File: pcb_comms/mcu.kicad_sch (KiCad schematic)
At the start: 24 parts, among them SW1 SW_SPDT, U3 STM32WLE5CCU6, Y2 32MHz

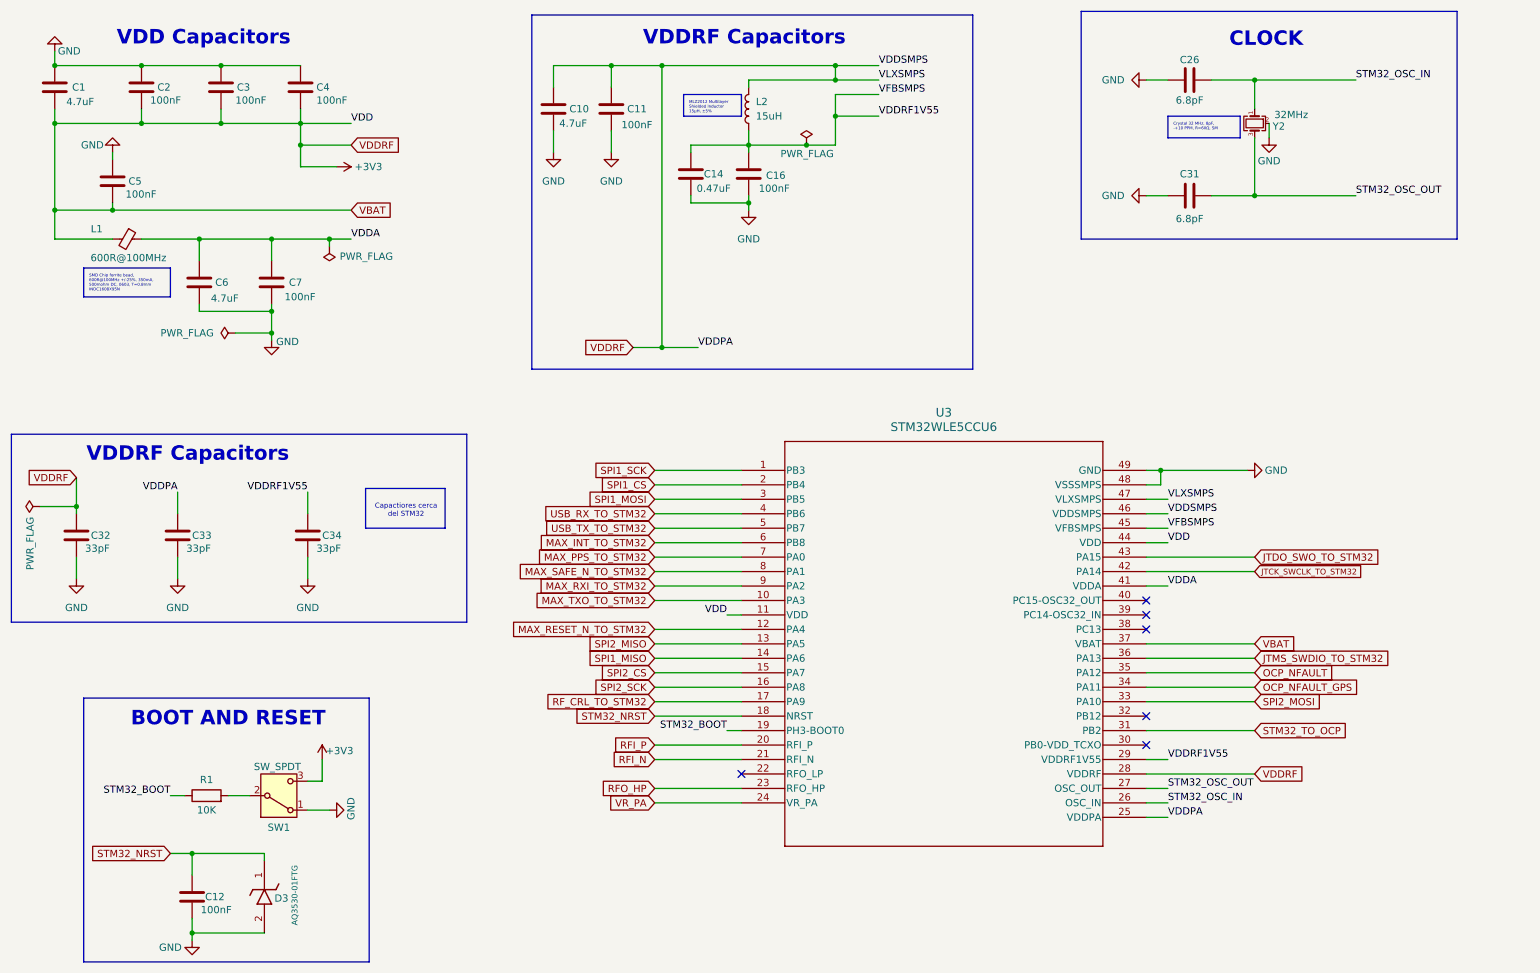
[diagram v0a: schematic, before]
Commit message: Version 1.0. No DRA yet
From now on I will make the connections for IIS and then adapt it for the club
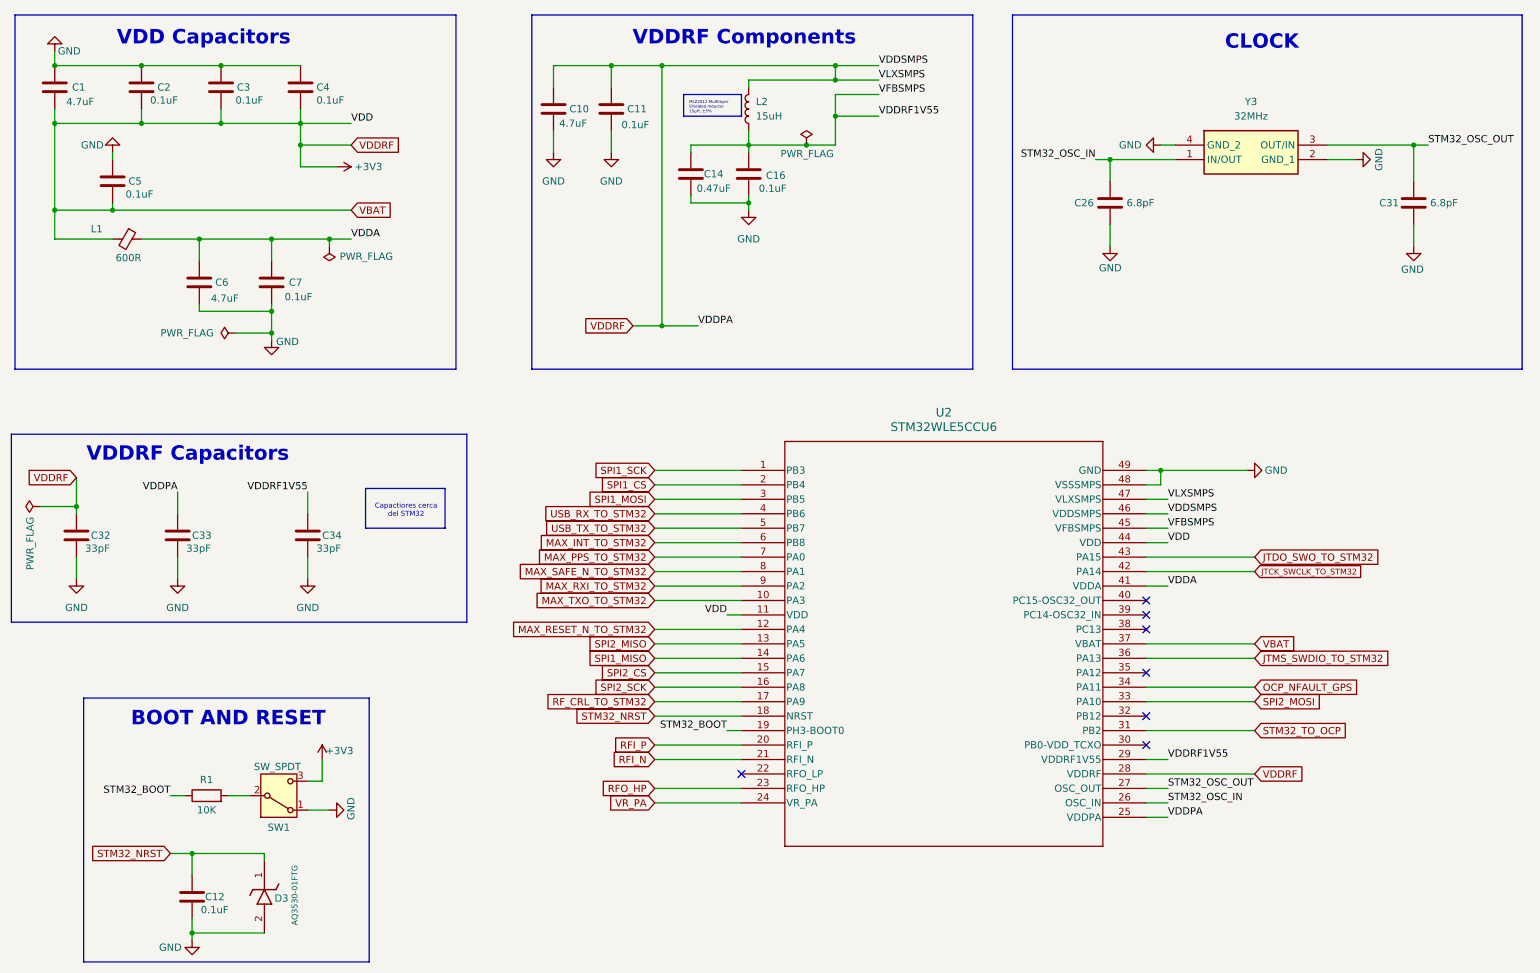
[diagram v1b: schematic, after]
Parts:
- removed U3: STM32WLE5CCU6, symbol STM32WL5:STM32WLE5CCU6
- removed Y2: 32MHz, symbol Device:Crystal_GND24_Small
- added U2: STM32WLE5CCU6, STM32WLE5:UFQFPN48_STM, symbol STM32WLE5:STM32WLE5CCU6
- added Y3: 32MHz, STM32WLE5_Crystal_32MHz:STM32WLE5_Crystal_32MHz_ECS320837CKMTR3, symbol STM32WLE5_Crystal_32MHz_ECS-320-8-37-CKM-TR3:ECS-320-8-37-CKM-TR3
- C11, C12, C16, C2, C3, C4, C5, C7: value 100nF -> 0.1uF
- L1: value 600R@100MHz -> 600R
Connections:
- net +3V3: now also U2.11 (VDD), U2.25 (VDDPA), U2.28 (VDDRF), U2.37 (VBAT), U2.44 (VDD), U2.46 (VDDSMPS), U2.47 (VLXSMPS)
- net GND: now also U2.48 (VSSSMPS), U2.49 (GND), Y3.2 (GND_1), Y3.4 (GND_2)
- net JTCK_SWCLK_TO_STM32: now also U2.42 (PA14)
- net JTDO_SWO_TO_STM32: now also U2.43 (PA15)
- net JTMS_SWDIO_TO_STM32: now also U2.36 (PA13)
- net MAX_INT_TO_STM32: now also U2.6 (PB8)
- net MAX_PPS_TO_STM32: now also U2.7 (PA0)
- net MAX_RESET_N_TO_STM32: now also U2.12 (PA4)
- net MAX_RXI_TO_STM32: now also U2.9 (PA2)
- net MAX_SAFE_N_TO_STM32: now also U2.8 (PA1)
- net MAX_TXO_TO_STM32: now also U2.10 (PA3)
- net OCP_NFAULT_GPS: now also U2.34 (PA11)
- net RFI_N: now also U2.21 (RFI_N)
- net RFI_P: now also U2.20 (RFI_P)
- net RFO_HP: now also U2.23 (RFO_HP)
- net RF_CRL_TO_STM32: now also U2.17 (PA9)
- net SPI1_CS: now also U2.2 (PB4)
- net SPI1_MISO: now also U2.14 (PA6)
- net SPI1_MOSI: now also U2.3 (PB5)
- net SPI1_SCK: now also U2.1 (PB3)
- net SPI2_CS: now also U2.15 (PA7)
- net SPI2_MISO: now also U2.13 (PA5)
- net SPI2_MOSI: now also U2.33 (PA10)
- net SPI2_SCK: now also U2.16 (PA8)
- net STM32_BOOT: now also U2.19 (PH3-BOOT0)
- net STM32_NRST: now also U2.18 (NRST)
- net STM32_OSC_IN: now also U2.26 (OSC_IN), Y3.1 (IN/OUT)
- net STM32_OSC_OUT: now also U2.27 (OSC_OUT), Y3.3 (OUT/IN)
- net STM32_TO_OCP: now also U2.31 (PB2)
- net USB_RX_TO_STM32: now also U2.4 (PB6)
- net USB_TX_TO_STM32: now also U2.5 (PB7)
- net VDDA: now also U2.41 (VDDA)
- net VDDRF1V55: now also U2.29 (VDDRF1V55), U2.45 (VFBSMPS)
- net VR_PA: now also U2.24 (VR_PA)
- no-connect marks 6 -> 7
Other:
- note added: "VDDRF Components"
- moved on the sheet: C26, C31
